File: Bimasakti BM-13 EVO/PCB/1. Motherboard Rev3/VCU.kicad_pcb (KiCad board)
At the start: 2 copper layers, 184 x 205 mm, 30 parts, among them J1 6437288-3, J10 power, J11 6437288-3, J8 SIGNAL 1, J9 SIGNAL 2

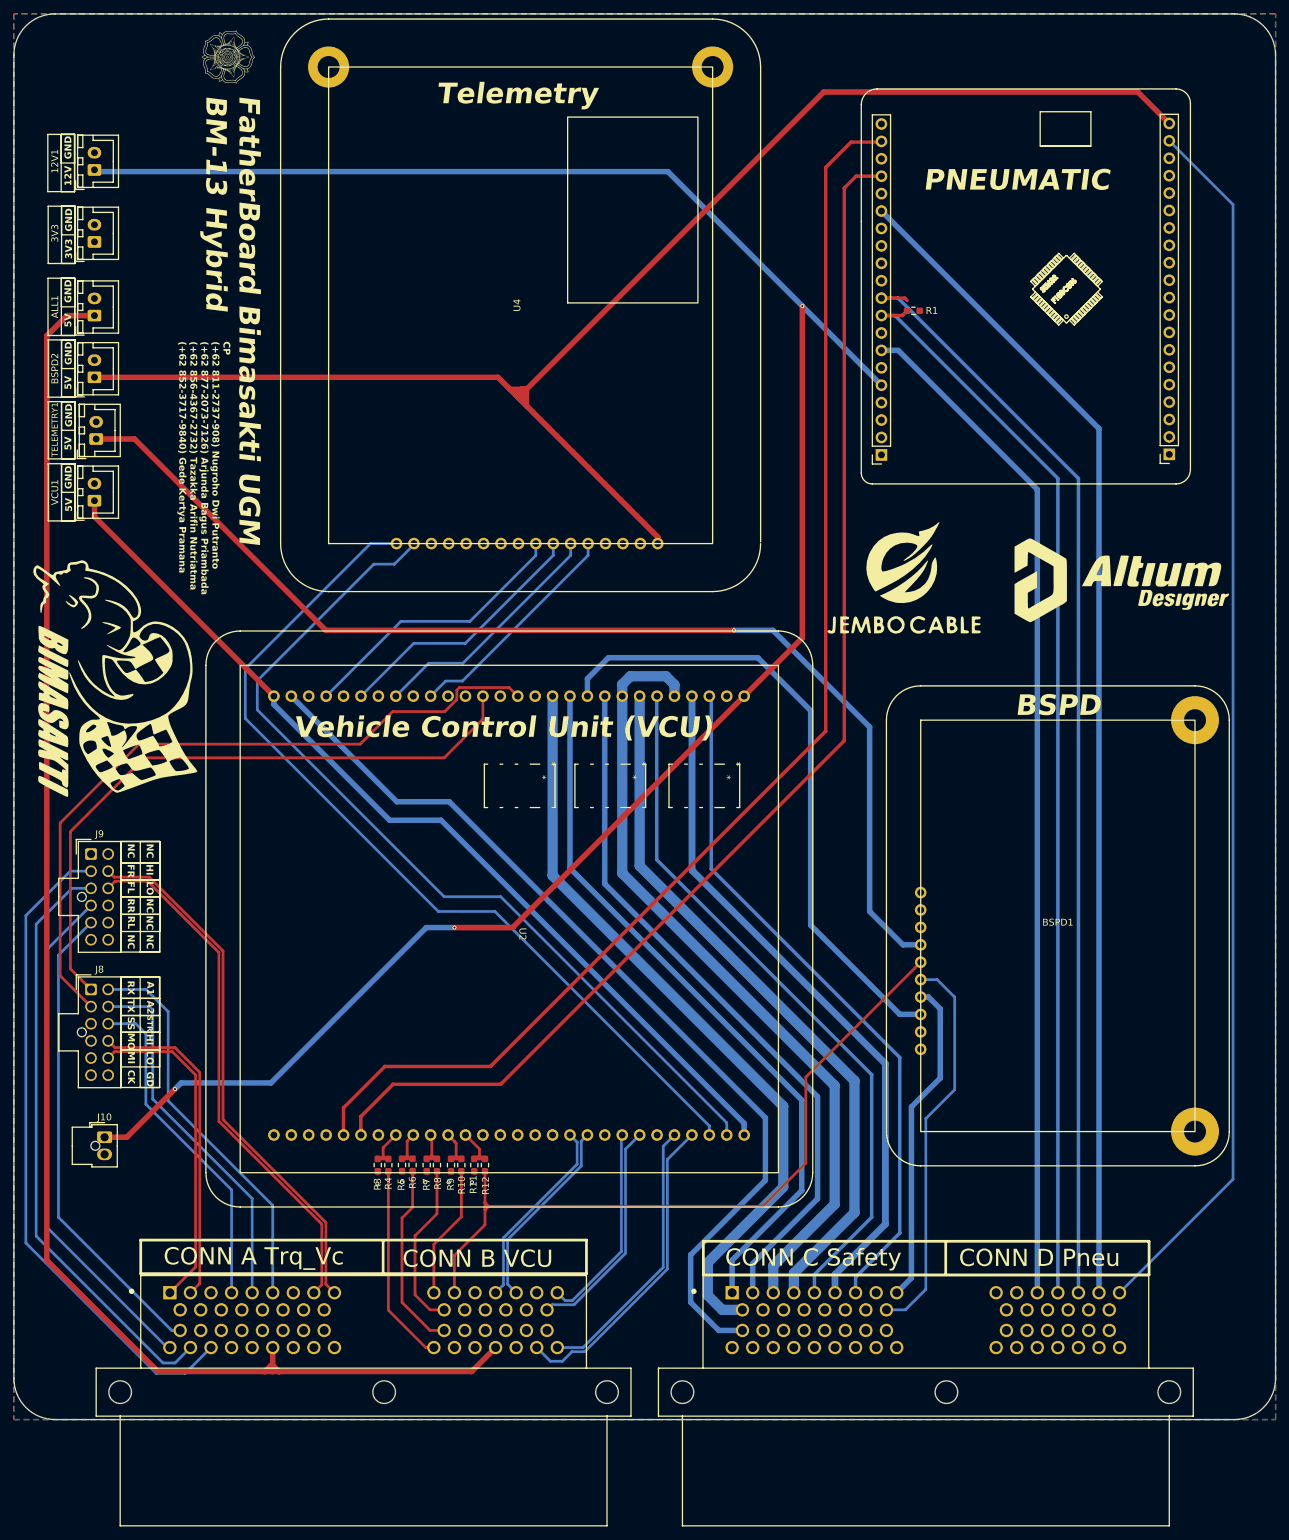
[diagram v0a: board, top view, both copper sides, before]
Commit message: rapiin
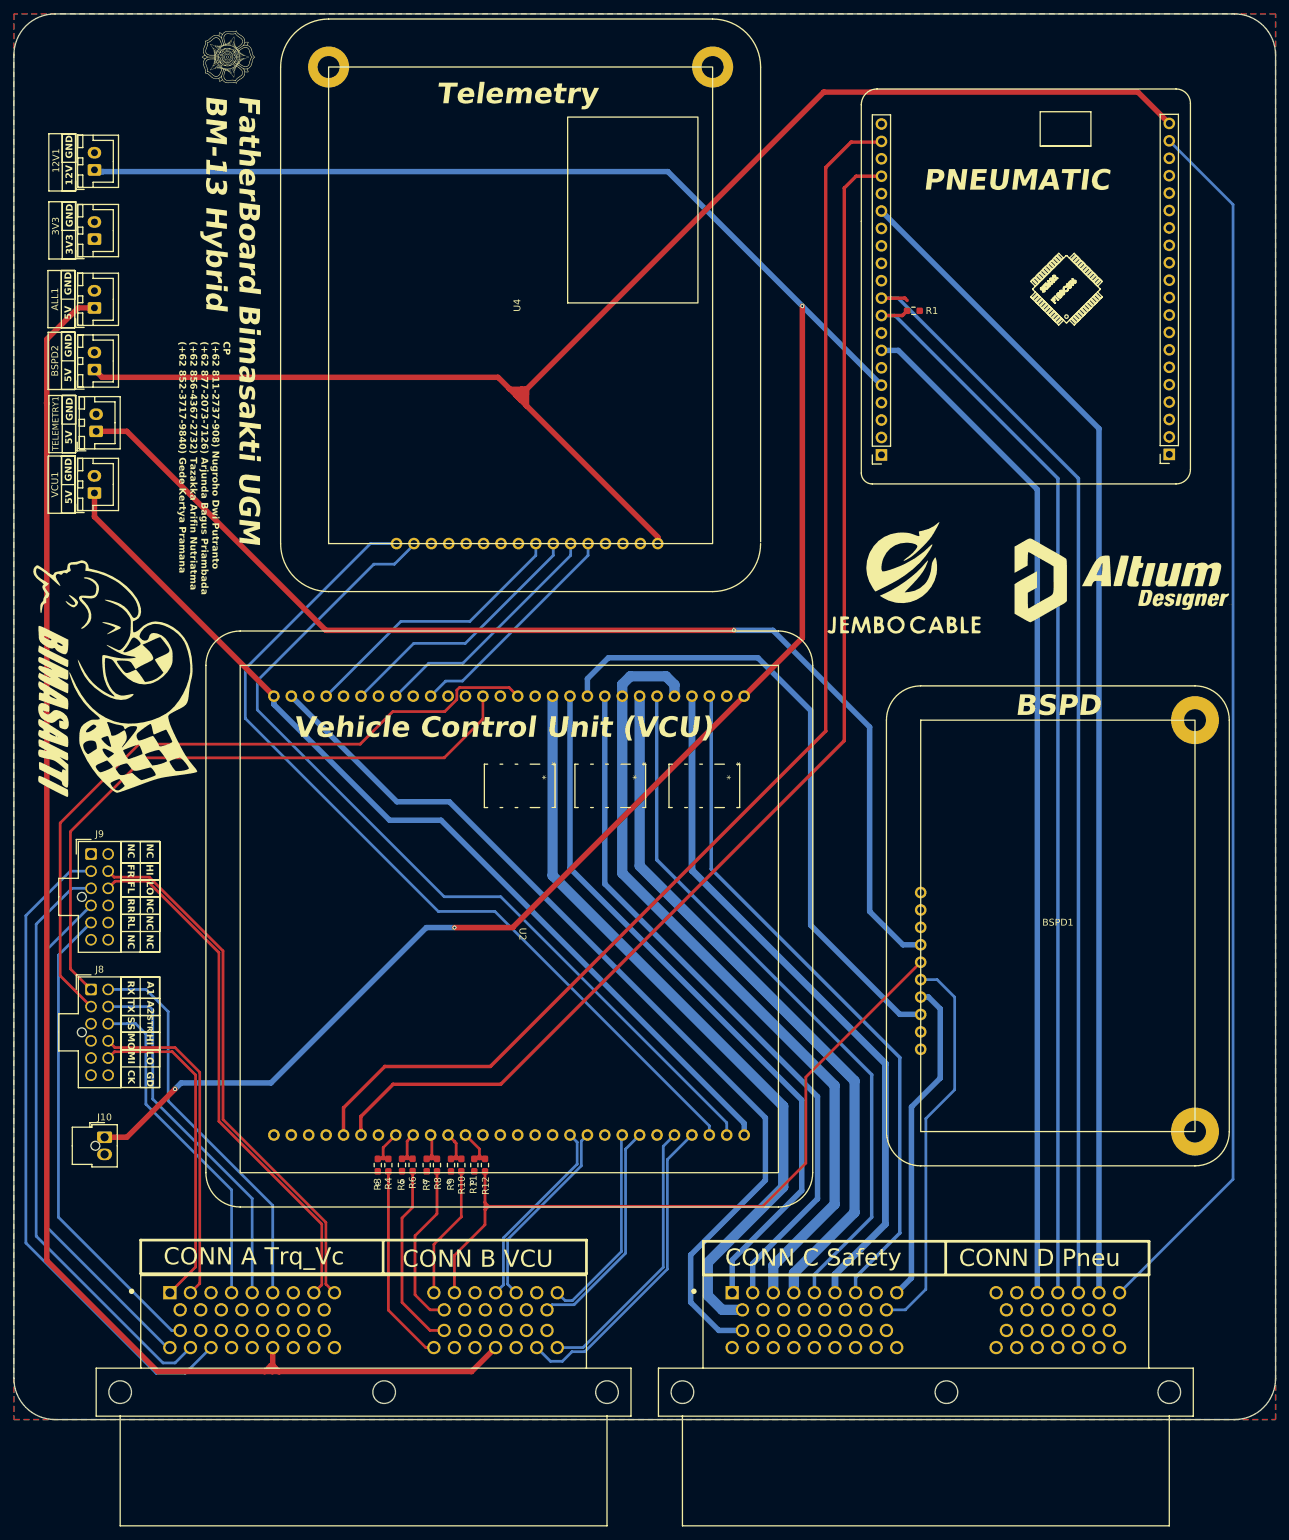
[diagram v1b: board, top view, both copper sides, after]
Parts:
- moved ALL1 1.12 mm to (175.7, 146.9)
- moved BSPD2 1.12 mm to (175.7, 155.9)
- moved TELEMETRY1 1.12 mm to (176.0, 164.9)
- moved VCU1 1.12 mm to (175.7, 173.9)
- moved 3V3 0.40 mm to (175.8, 136.8)
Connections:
- BSPD2 pad 1: 5V_B -> 5V_T
- TELEMETRY1 pad 1: 5V_T -> 5V_B
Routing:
- net 12V: track 308.0 -> 309.3 mm
- net 5V_V: track 136.1 -> 137.3 mm
